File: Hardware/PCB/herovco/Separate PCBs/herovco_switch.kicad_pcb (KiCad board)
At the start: 2 copper layers, 19 x 17 mm, 5 parts, among them J13 Wire pads, J14 Conn_01x01, J15 Conn_01x01, J16 Conn_01x01, SW2 SW_DP3T

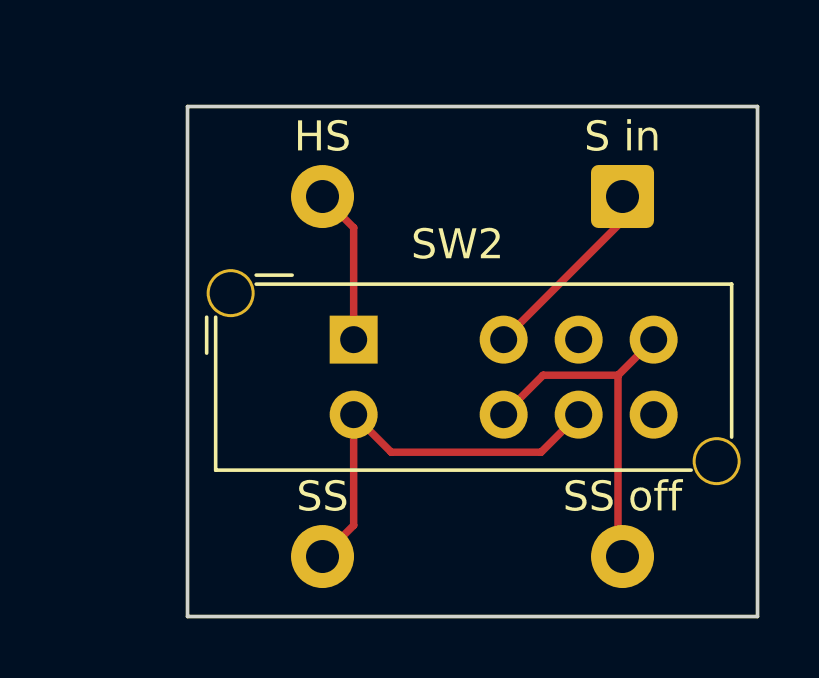
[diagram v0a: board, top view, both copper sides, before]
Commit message: Libraries, redo gerbers
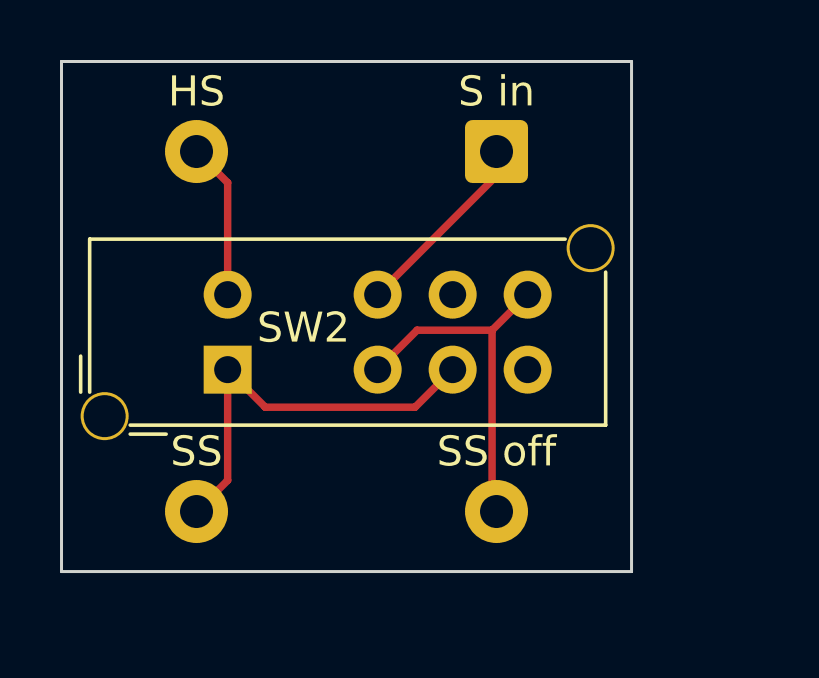
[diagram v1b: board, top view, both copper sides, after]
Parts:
- added B3: Board, ao_tht:Board_Marker, F.Cu at (147.8, 90.0)
- moved J13 4.46 mm to (150.8, 93.0)
- moved J14 4.46 mm to (150.8, 105.0)
- moved J15 4.46 mm to (140.8, 105.0)
- moved J16 4.46 mm to (140.8, 93.0)
- moved SW2 4.32 mm to (141.8, 100.3)
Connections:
- SW2 pad 1: Board_0-/Octave and sync switches/HARD_SYNCA_P -> Board_0-/Octave and sync switches/SOFT_SYNC_OFF_P
- SW2 pad 2: Board_0-/Octave and sync switches/SYNCA_P -> Board_0-/Octave and sync switches/SOFT_SYNCA_P
- SW2 pad 3: Board_0-unconnected-(SW2-Pad3) -> Board_0-/Octave and sync switches/SOFT_SYNC_OFF_P
- SW2 pad 4: Board_0-/Octave and sync switches/SOFT_SYNCA_P -> Board_0-unconnected-(SW2-Pad4)
- SW2 pad 5: Board_0-/Octave and sync switches/SOFT_SYNC_OFF_P -> Board_0-/Octave and sync switches/HARD_SYNCA_P
- SW2 pad 6: Board_0-/Octave and sync switches/SOFT_SYNCA_P -> Board_0-/Octave and sync switches/SYNCA_P
- SW2 pad 7: Board_0-/Octave and sync switches/SOFT_SYNC_OFF_P -> Board_0-unconnected-(SW2-Pad7)
- SW2 pad 8: Board_0-unconnected-(SW2-Pad8) -> Board_0-/Octave and sync switches/SOFT_SYNCA_P
